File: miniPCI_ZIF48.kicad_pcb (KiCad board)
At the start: 2 copper layers, 61.5 x 50.9 mm, 6 parts

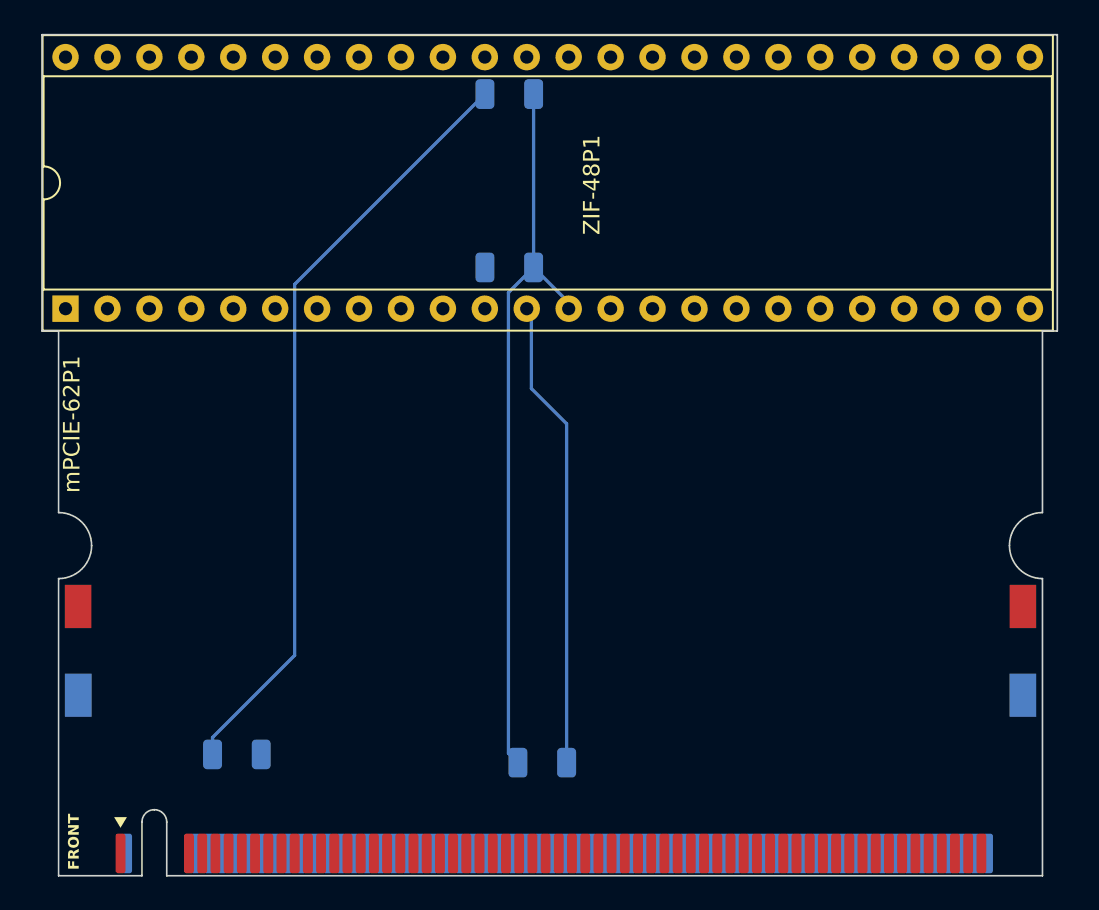
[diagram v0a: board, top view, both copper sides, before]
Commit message: Passed all DRCs/PCB_Editor
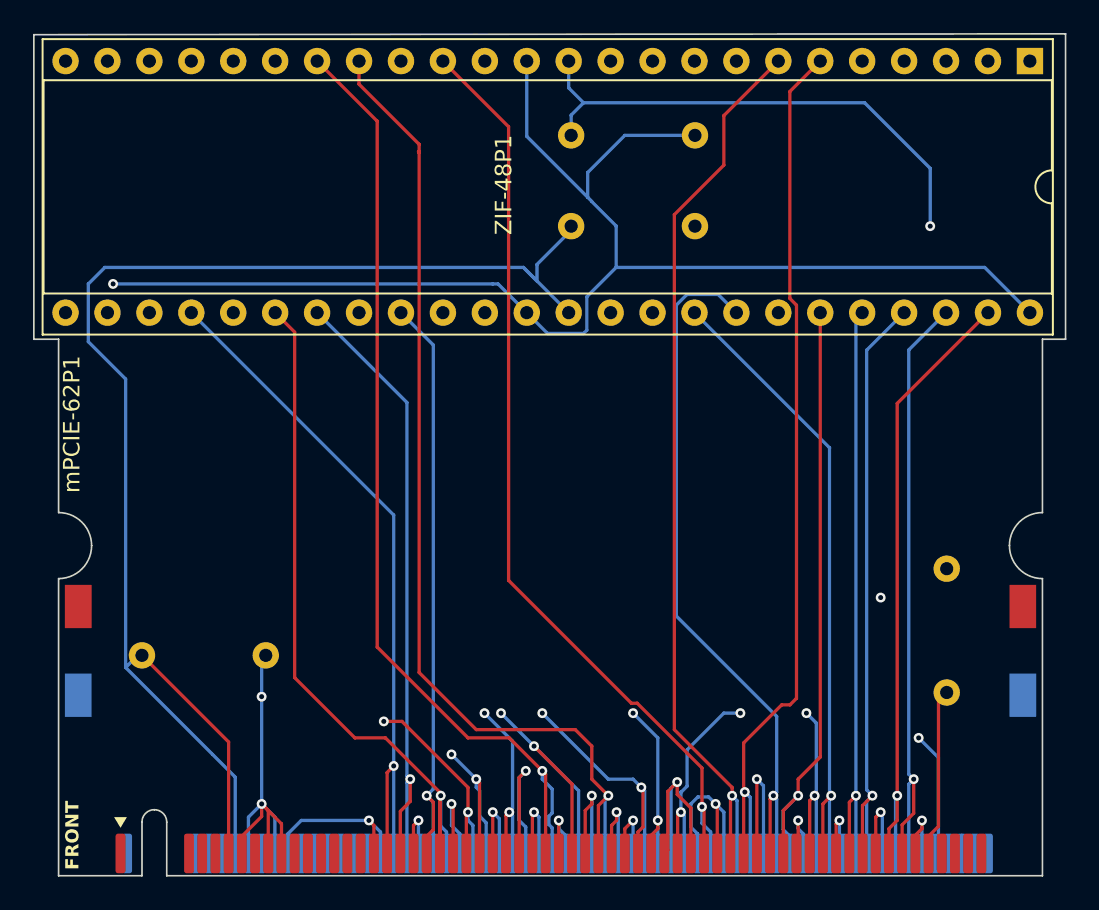
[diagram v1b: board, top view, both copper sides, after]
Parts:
- C1, C2, C3, C4: footprint Capacitor_SMD:C_1206_3216Metric -> Capacitor_THT:C_Axial_L3.8mm_D2.6mm_P7.50mm_Horizontal
- moved ZIF-48P1 60.3 mm to (194.0, 90.5), turned to -90 degrees
- moved C2 27.2 mm to (189.0, 121.2), turned to -90 degrees
- moved C1 8.84 mm to (166.2, 95.0)
- moved C4 8.84 mm to (166.2, 100.5)
- moved C3 6.25 mm to (147.8, 126.5)
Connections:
- mPCIE-62P1 pad 10: GND -> unconnected-(mPCIE-62P1-NO-Pad10)_1
- mPCIE-62P1 pad 11: unconnected-(ZIF-48P1-Pad11) -> unconnected-(mPCIE-62P1-CE4-Pad11)_1
- mPCIE-62P1 pad 2: unconnected-(ZIF-48P1-Pad2) -> unconnected-(mPCIE-62P1-3.3V-Pad2)
- mPCIE-62P1 pad 3: unconnected-(ZIF-48P1-Pad3) -> unconnected-(mPCIE-62P1-VCC-Pad3)_1
- mPCIE-62P1 pad 4: unconnected-(ZIF-48P1-Pad4) -> unconnected-(mPCIE-62P1-VEXT-Pad4)
- mPCIE-62P1 pad 7: (no net) -> unconnected-(mPCIE-62P1-NO-Pad7)
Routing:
- net GND: track 44.8 -> 269.1 mm, vias 0 -> 19
- net ALE: track 0.00 -> 61.6 mm, vias 0 -> 1
- net WE: track 0.00 -> 60.6 mm, vias 0 -> 1
- net V2-58: track 28.4 -> 88.9 mm, vias 0 -> 2
- net CLE: track 0.00 -> 60.1 mm, vias 0 -> 2
- net CE3: track 0.00 -> 57.8 mm, vias 0 -> 1
- net CE2: track 0.00 -> 57.6 mm, vias 0 -> 2
- net RB1: track 0.00 -> 55.7 mm, vias 0 -> 1
- net RE: track 0.00 -> 54.9 mm, vias 0 -> 2
- net CE0: track 0.00 -> 54.5 mm, vias 0 -> 1
- net RB2: track 0.00 -> 54.4 mm, vias 0 -> 1
- net CE1: track 0.00 -> 51.3 mm, vias 0 -> 2
- net D9: track 0.00 -> 46.1 mm, vias 0 -> 2
- net D0: track 0.00 -> 45.9 mm, vias 0 -> 1
- net D1: track 0.00 -> 45.1 mm, vias 0 -> 1
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- added copper zone on In2.Cu, net GND
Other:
- board size 61.5 x 50.9 mm -> 62.5 x 51 mm
- copper layers 2 -> 4
